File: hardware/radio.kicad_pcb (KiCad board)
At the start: 2 copper layers, 65 x 56 mm, 89 parts, among them J1 JCLK, U1 G144A12, U3V3t1V8 NCP1117ST18T3G, U5V0t3V3 NCP1117ST33T3G

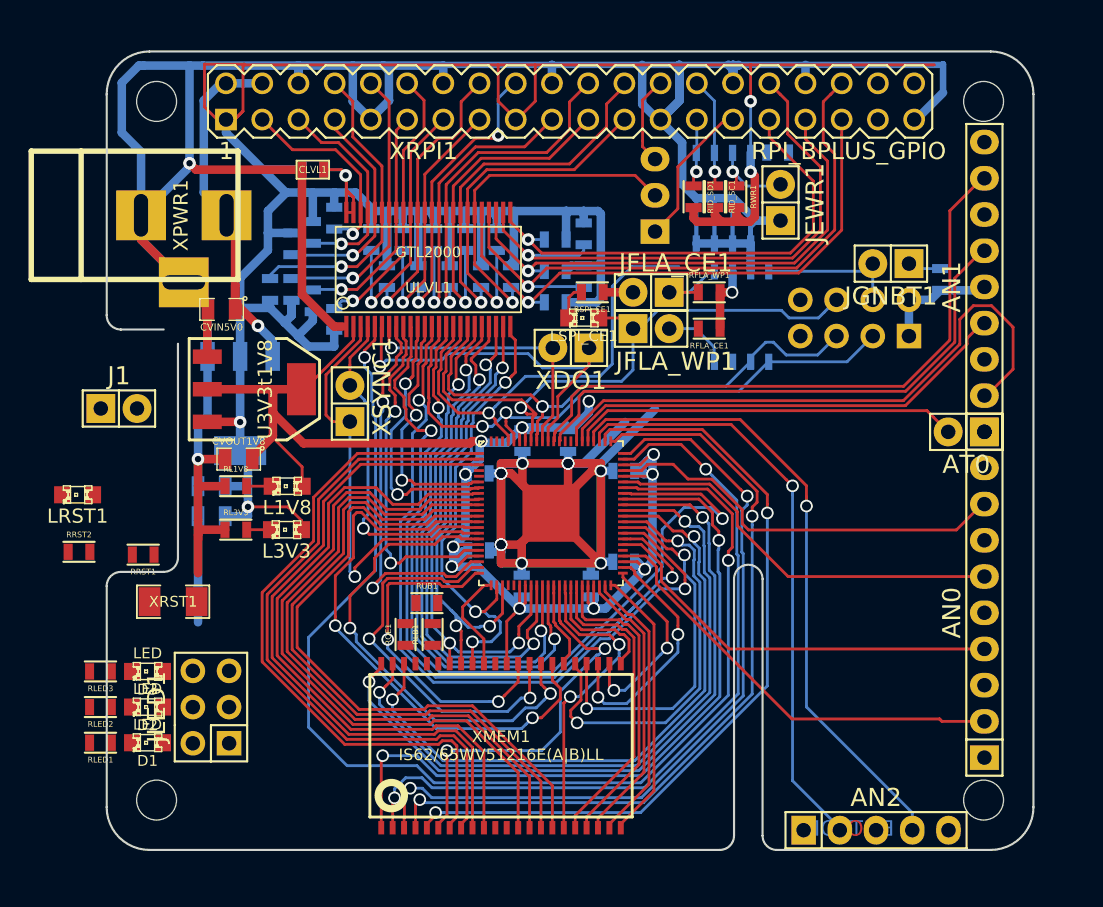
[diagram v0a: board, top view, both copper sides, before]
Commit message: All traces routed I think.
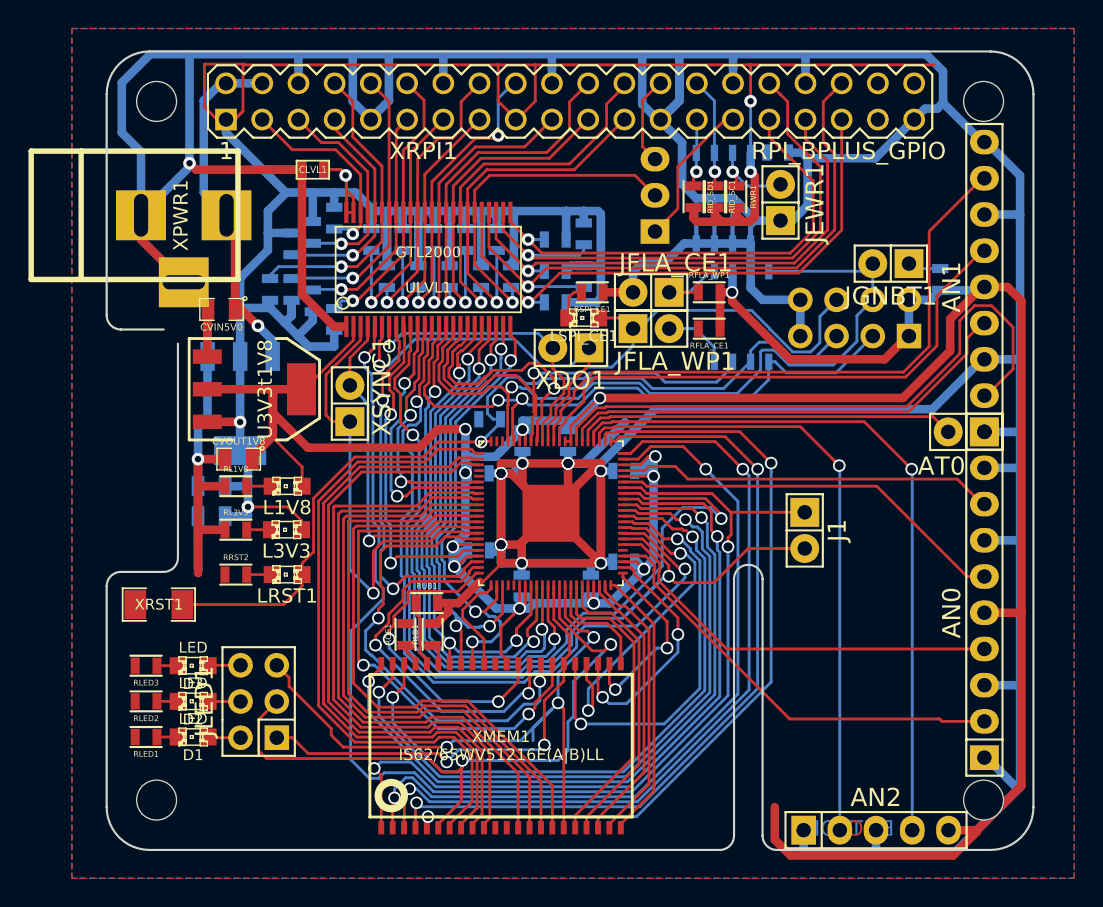
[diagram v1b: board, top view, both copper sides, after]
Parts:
- RRST1: moved to B.Cu
- moved J1 48.9 mm to (65.9, 50.9), turned to 270 degrees
- moved RRST1 26.1 mm to (43.8, 43.1), turned to 0 degrees
- moved LRST1 15.7 mm to (29.6, 54.0)
- moved RRST2 11.1 mm to (26.0, 54.0)
- moved JLED1 3.37 mm to (27.6, 62.9)
- moved D1 3.22 mm to (23.0, 65.4)
- moved RLED1 3.22 mm to (19.7, 65.4)
- moved D2 3.22 mm to (23.0, 62.9)
- moved D3 3.22 mm to (23.0, 60.4)
- moved RLED2 3.22 mm to (19.7, 62.9)
- moved RLED3 3.22 mm to (19.7, 60.4)
- moved XRST1 1.02 mm to (20.6, 56.1), turned to 180 degrees
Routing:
- net GND: track 365.1 -> 490.2 mm
- net VDD: track 128.1 -> 244.2 mm
- net RST: track 0.00 -> 53.2 mm, vias 0 -> 1
- net /ADDRN18: track 6.13 -> 32.4 mm, vias 0 -> 2
- net /~WE: track 21.8 -> 46.1 mm, vias 2 -> 3
- net /~CE: track 27.9 -> 47.8 mm
- net SPI_MISO: track 42.6 -> 55.6 mm
- net REFCLK2_L: track 55.9 -> 67.1 mm
- net /DATA7: track 46.1 -> 40.3 mm
- net /DATA6: track 46.5 -> 41.2 mm
- net /DATA5: track 46.9 -> 41.6 mm
- net /DATA4: track 47.3 -> 42.2 mm
- net /717.ao: track 45.1 -> 50.0 mm
- net Net-(RUB1-Pad2): track 0.00 -> 4.56 mm
- net /DATA3: track 46.8 -> 42.4 mm
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- added copper zone on B.Cu, net GND
- added copper zone on F.Cu, net VDD

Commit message: Lots of small fixes.
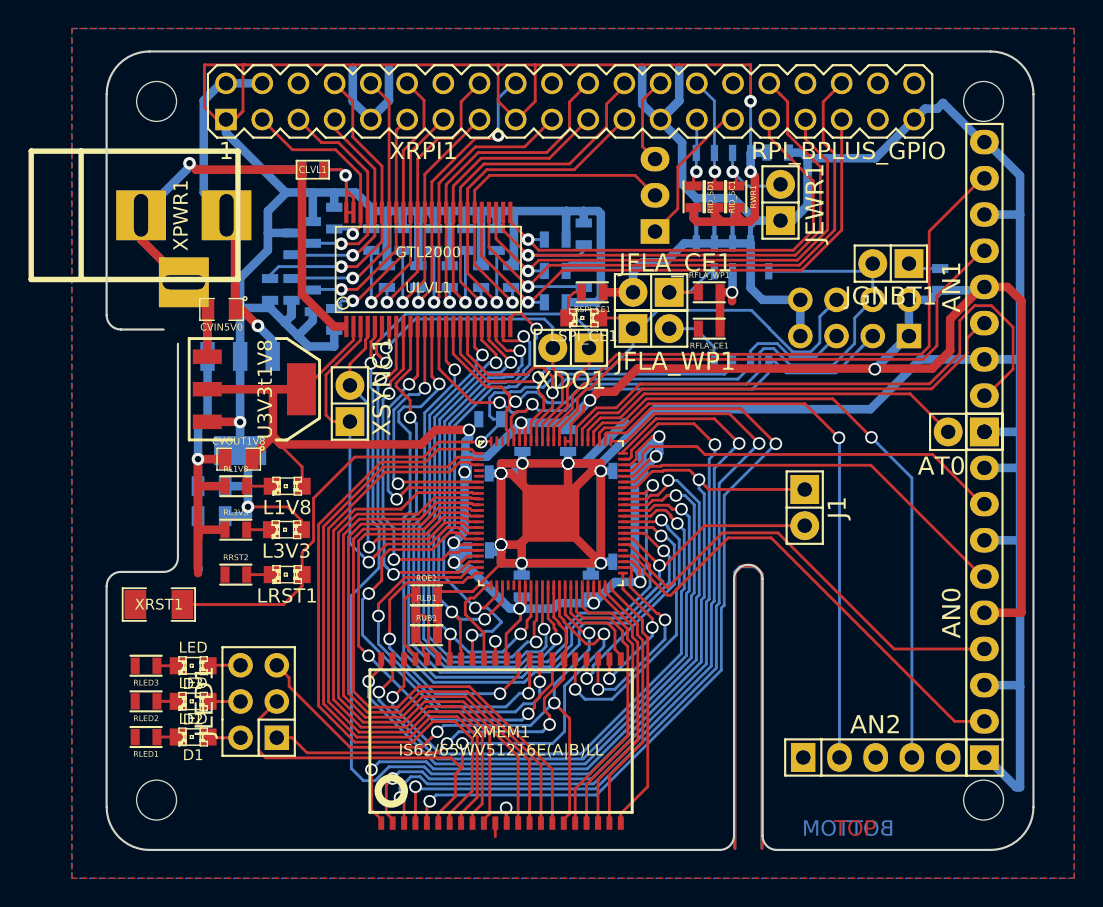
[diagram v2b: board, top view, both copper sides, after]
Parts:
- moved AN2 5.10 mm to (70.9, 66.8)
- moved ROE1 3.12 mm to (39.4, 55.5), turned to 180 degrees
- moved RUB1 2.25 mm to (39.4, 58.2)
- moved J1 1.60 mm to (65.9, 49.3)
- moved RLB1 1.41 mm to (39.4, 56.9), turned to 180 degrees
- moved XMEM1 0.33 mm to (44.6, 65.7)
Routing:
- net GND: track 490.2 -> 375.4 mm, vias 12 -> 14
- net (no net): track 0.00 -> 81.8 mm
- net VDD: track 244.2 -> 200.1 mm, vias 12 -> 13
- net +3.3V: track 222.0 -> 209.5 mm
- net /GPIO_25_L: track 60.8 -> 54.1 mm
- net /ADDR8: track 29.4 -> 22.8 mm
- net /ADDR9: track 23.1 -> 17.4 mm
- net SPI_~CE: track 48.5 -> 43.4 mm
- net /ADDR7: track 46.8 -> 42.0 mm
- net /ADDR6: track 49.2 -> 44.5 mm
- net /SDA1_L: track 32.8 -> 28.4 mm
- net /ADDR5: track 51.3 -> 47.0 mm
- net /717.ao: track 50.0 -> 45.9 mm
- net GPIO_06_L: track 32.8 -> 36.8 mm
- net SPI_CLK: track 40.9 -> 36.9 mm
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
